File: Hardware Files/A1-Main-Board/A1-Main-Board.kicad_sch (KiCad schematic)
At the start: 1 part

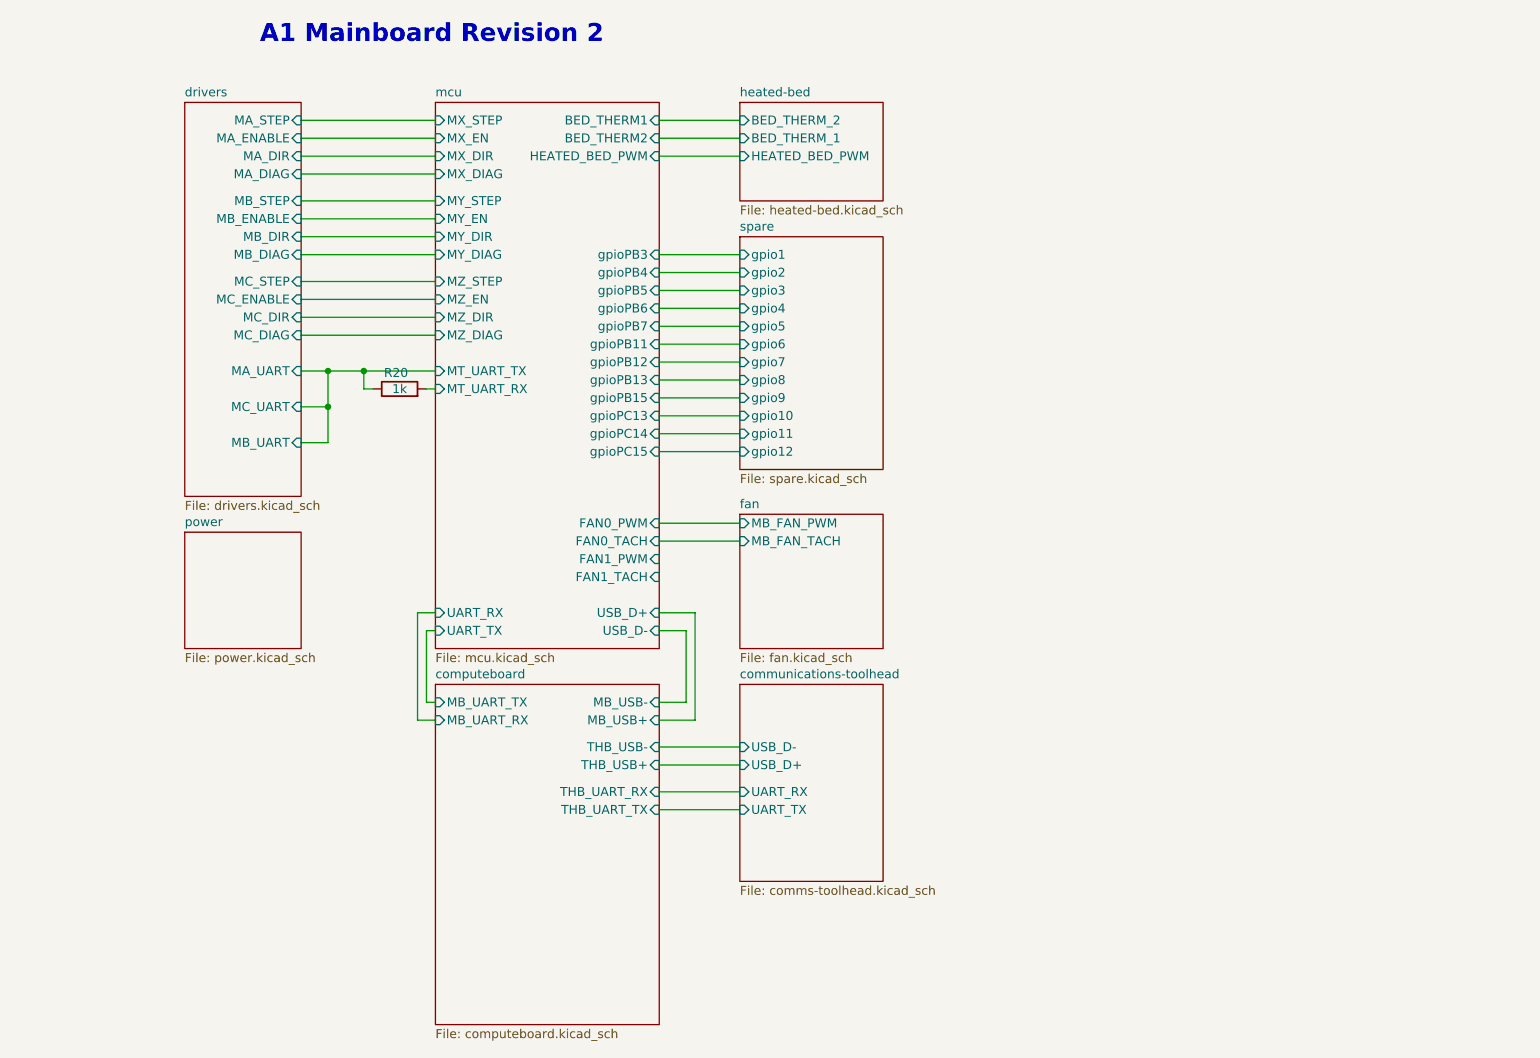
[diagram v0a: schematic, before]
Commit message: e
e
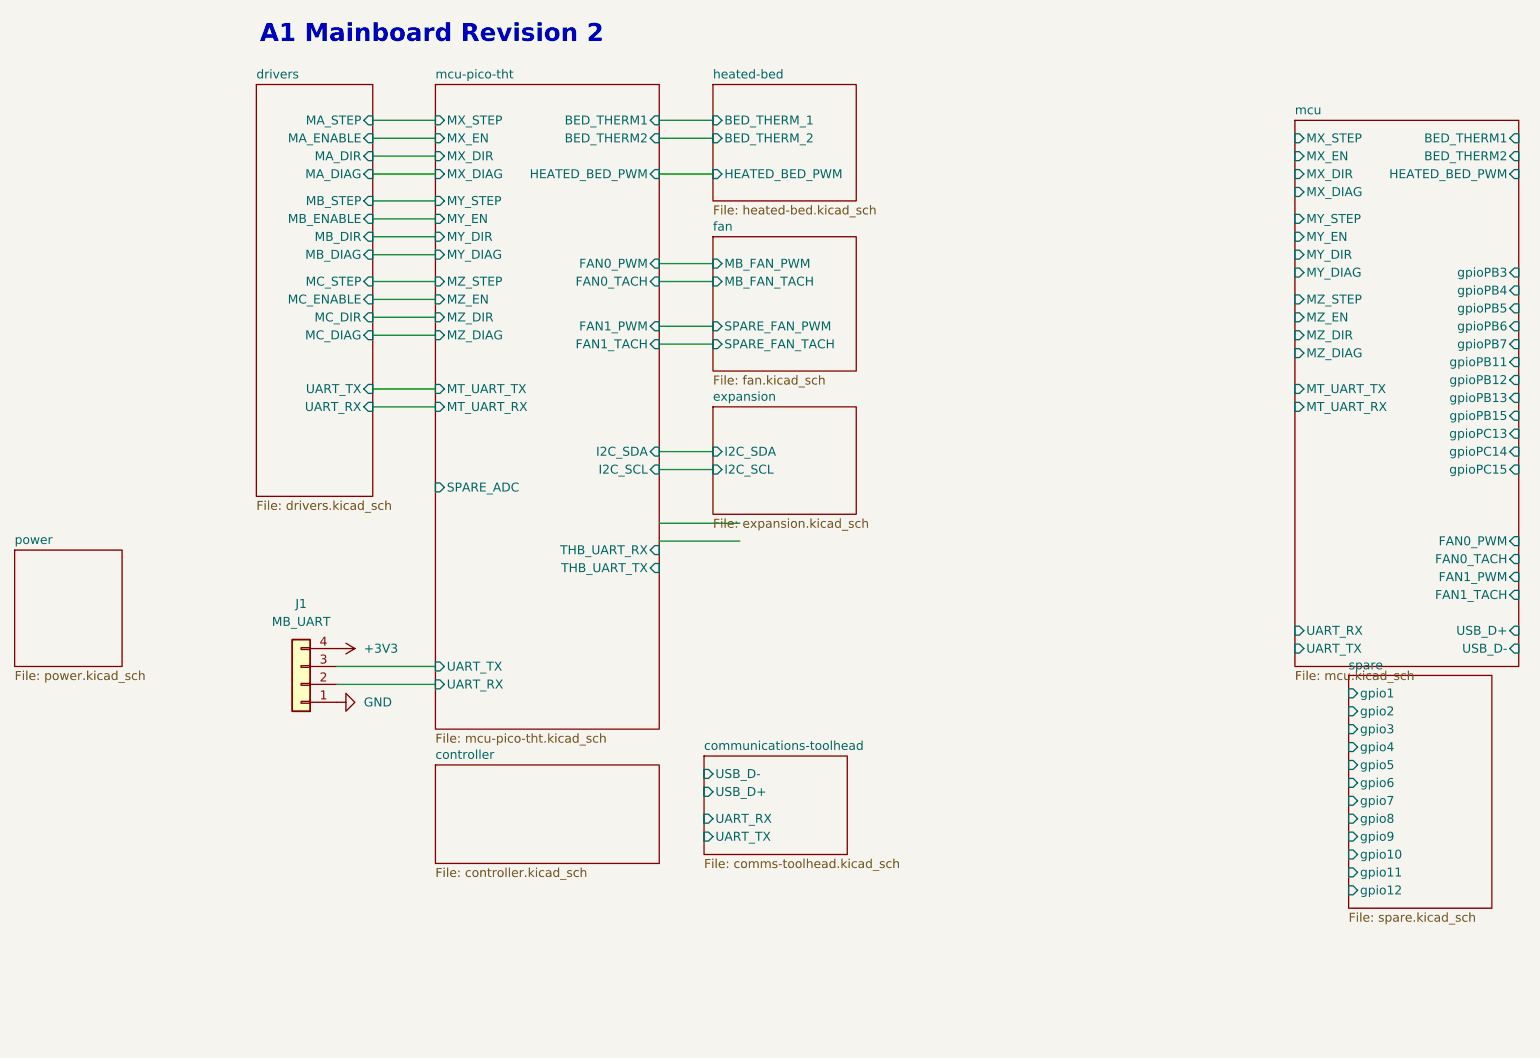
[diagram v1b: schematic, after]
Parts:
- removed R20: 1k, symbol Device:R
- added J1: MB_UART, Connector_JST:JST_XH_B4B-XH-A_1x04_P2.50mm_Vertical, symbol Connector_Generic:Conn_01x04
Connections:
- new net +3V3: J1.4 (Pin_4)
- new net GND: J1.1 (Pin_1)
- new net mcu-pico-tht/UART_RX: J1.2 (Pin_2)
- new net mcu-pico-tht/UART_TX: J1.3 (Pin_3)
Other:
- removed sheet computeboard
- added sheet controller (controller.kicad_sch)
- added sheet expansion (expansion.kicad_sch)
- added sheet mcu-pico-tht (mcu-pico-tht.kicad_sch)
- sheet drivers ports: added UART_RX, UART_TX; removed MA_UART, MB_UART, MC_UART
- sheet fan ports: added SPARE_FAN_PWM, SPARE_FAN_TACH; removed none
